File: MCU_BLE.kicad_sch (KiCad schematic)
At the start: 39 parts, among them Q1 DMG1012T, U1 STM32WB55RGVx, U3 AT25SL321-U, Y1 32MHz, Y2 32.768k

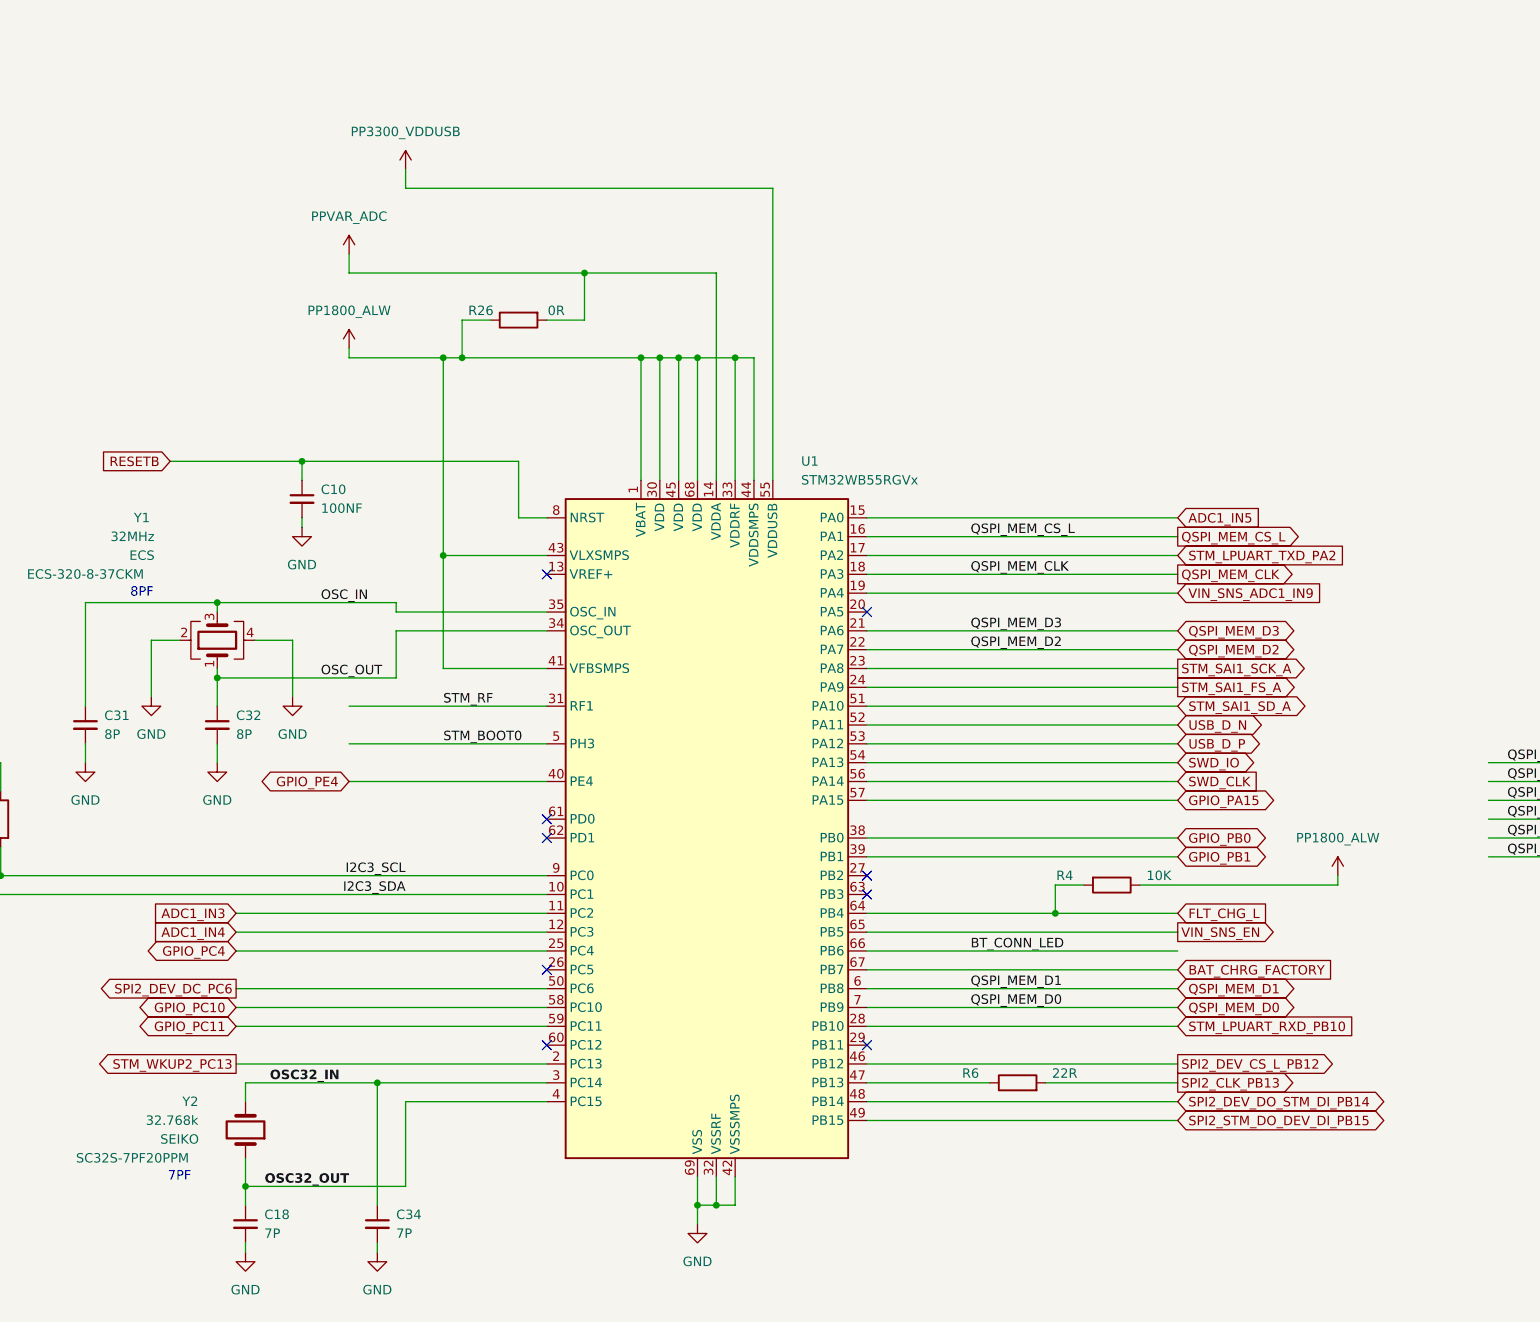
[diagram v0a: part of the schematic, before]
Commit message: updating design files
updating schematics, gerbers, design files, etc.
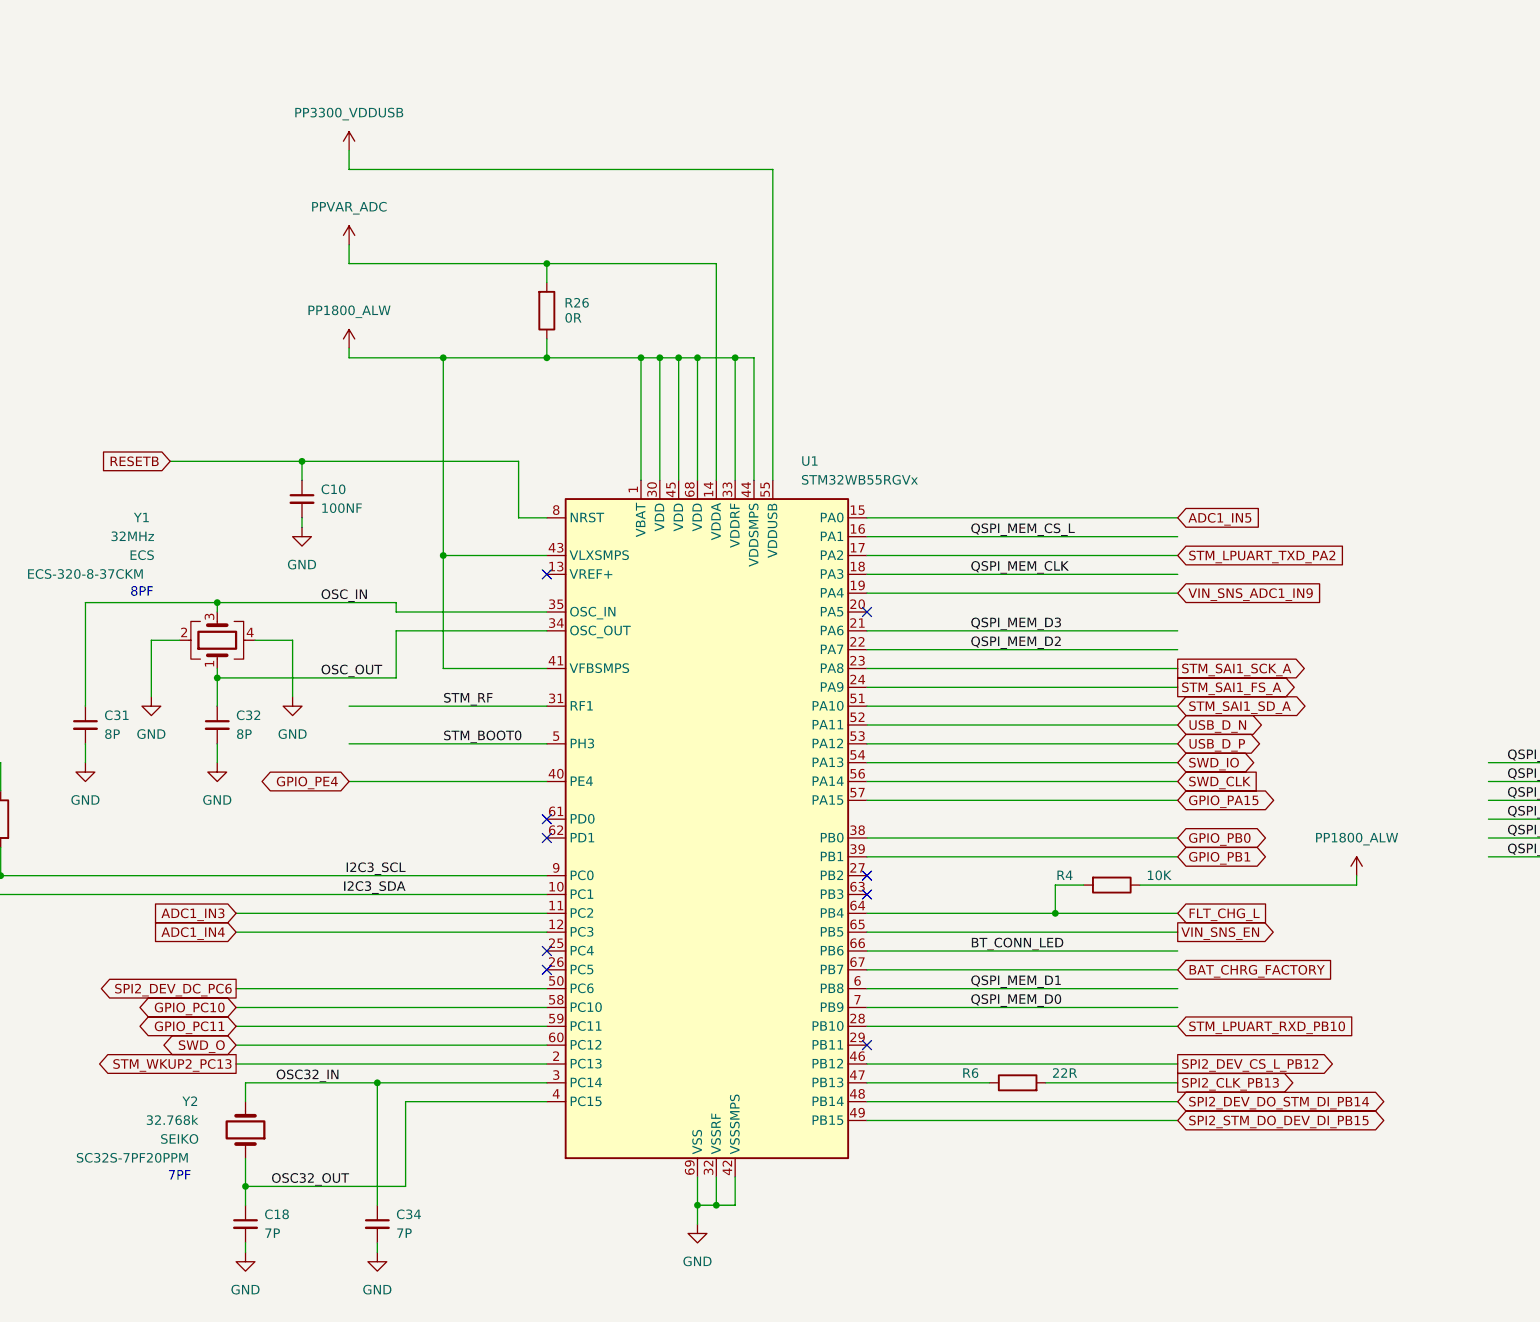
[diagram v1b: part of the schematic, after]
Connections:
- net SWD_O: now reaches U1.60 (PC12)
- net GPIO_PC4: no longer names the net of U1.25 (PC4)
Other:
- moved on the sheet: R26
